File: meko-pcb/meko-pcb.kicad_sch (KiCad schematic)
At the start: 208 parts, among them IC2 TPS7A2033PDBVR, IC4 TAD5212IRGER, IC5 AS5600-ASOM, J1 USB_C_Receptacle_USB2.0_16P, J2 Conn_ARM_JTAG_SWD_10, J3 GDEY0154D67, J5 503398-1892, Q1 SS8050, Q2 Si1308EDL, SW1 SW_Push, SW2 SW_Push, SW3 SW_Push, SW4 SW_Push, SW5 SW_Push, SW6 SW_Push, SW7 SW_Push, SW9 SW_Push, U1 nPM1300-QEXX, U2 nRF5340-QKxx, Y1 32MHz, Y2 32.768 kHz

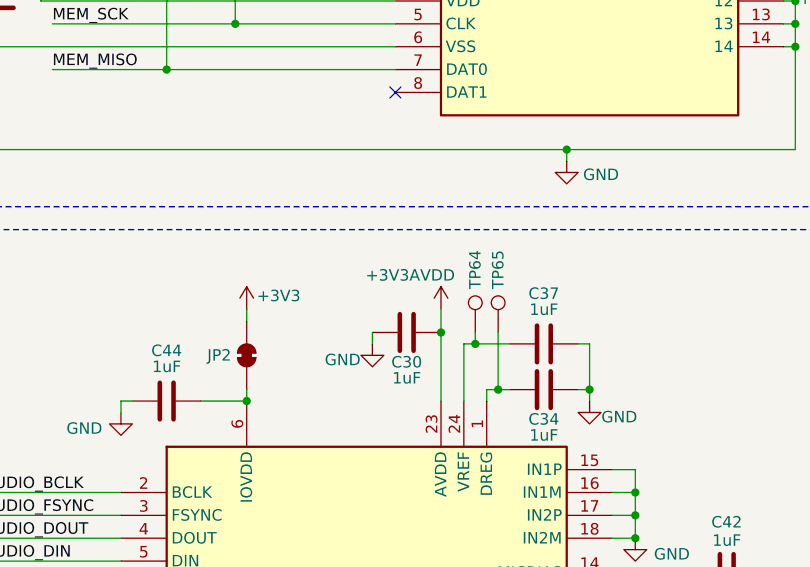
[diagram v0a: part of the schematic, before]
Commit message: made final changes
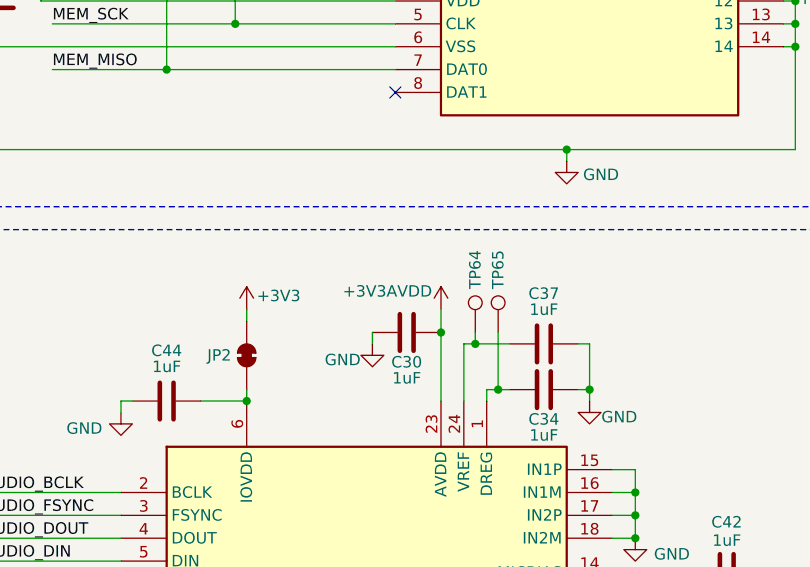
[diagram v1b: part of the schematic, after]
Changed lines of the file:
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@@
 	(wire
 		(pts
-			(xy 177.8 275.59) (xy 234.95 275.59)
-		)
-		(stroke
-			(width 0)
-			(type default)
-		)
-	)
-	(wire
-		(pts
 			(xy 157.48 275.59) (xy 166.37 275.59)
 		)
@@
 	(wire
 		(pts
+			(xy 177.8 275.59) (xy 234.95 275.59)
+		)
+		(stroke
+			(width 0)
+			(type default)
+		)
+	)
+	(wire
+		(pts
 			(xy 370.84 354.33) (xy 386.08 354.33)
 		)
@@
 		)
 		(property "Value" "+3V3AVDD"
-			(at 295.148 134.62 0)
+			(at 292.608 136.398 0)
 			(effects
 				(font
